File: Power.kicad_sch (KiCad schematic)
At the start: 39 parts, among them IC1 ADP2301AUJZ-R7, IC2 ADP2301AUJZ-R7, Q1 AO3401A, U1 LM2842X, U6 XT30PW-F, U7 XT30PW-M, U9 LP5907QMFX-3.3Q1

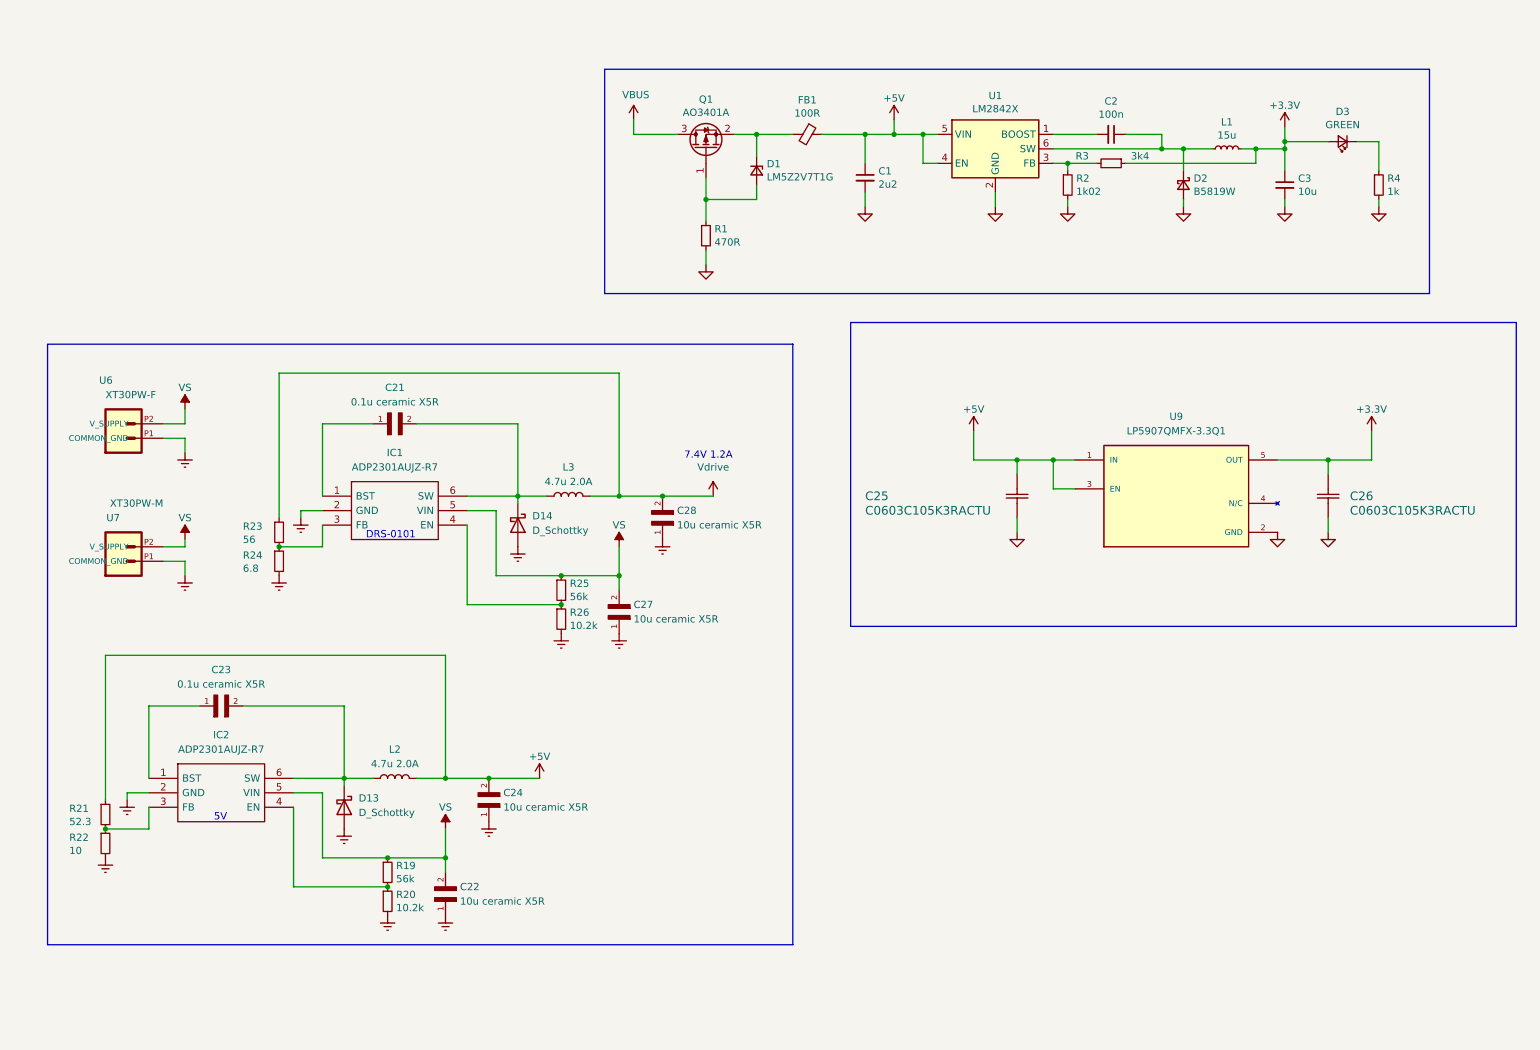
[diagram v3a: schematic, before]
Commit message: WEBGIOWEBGIOBWEG
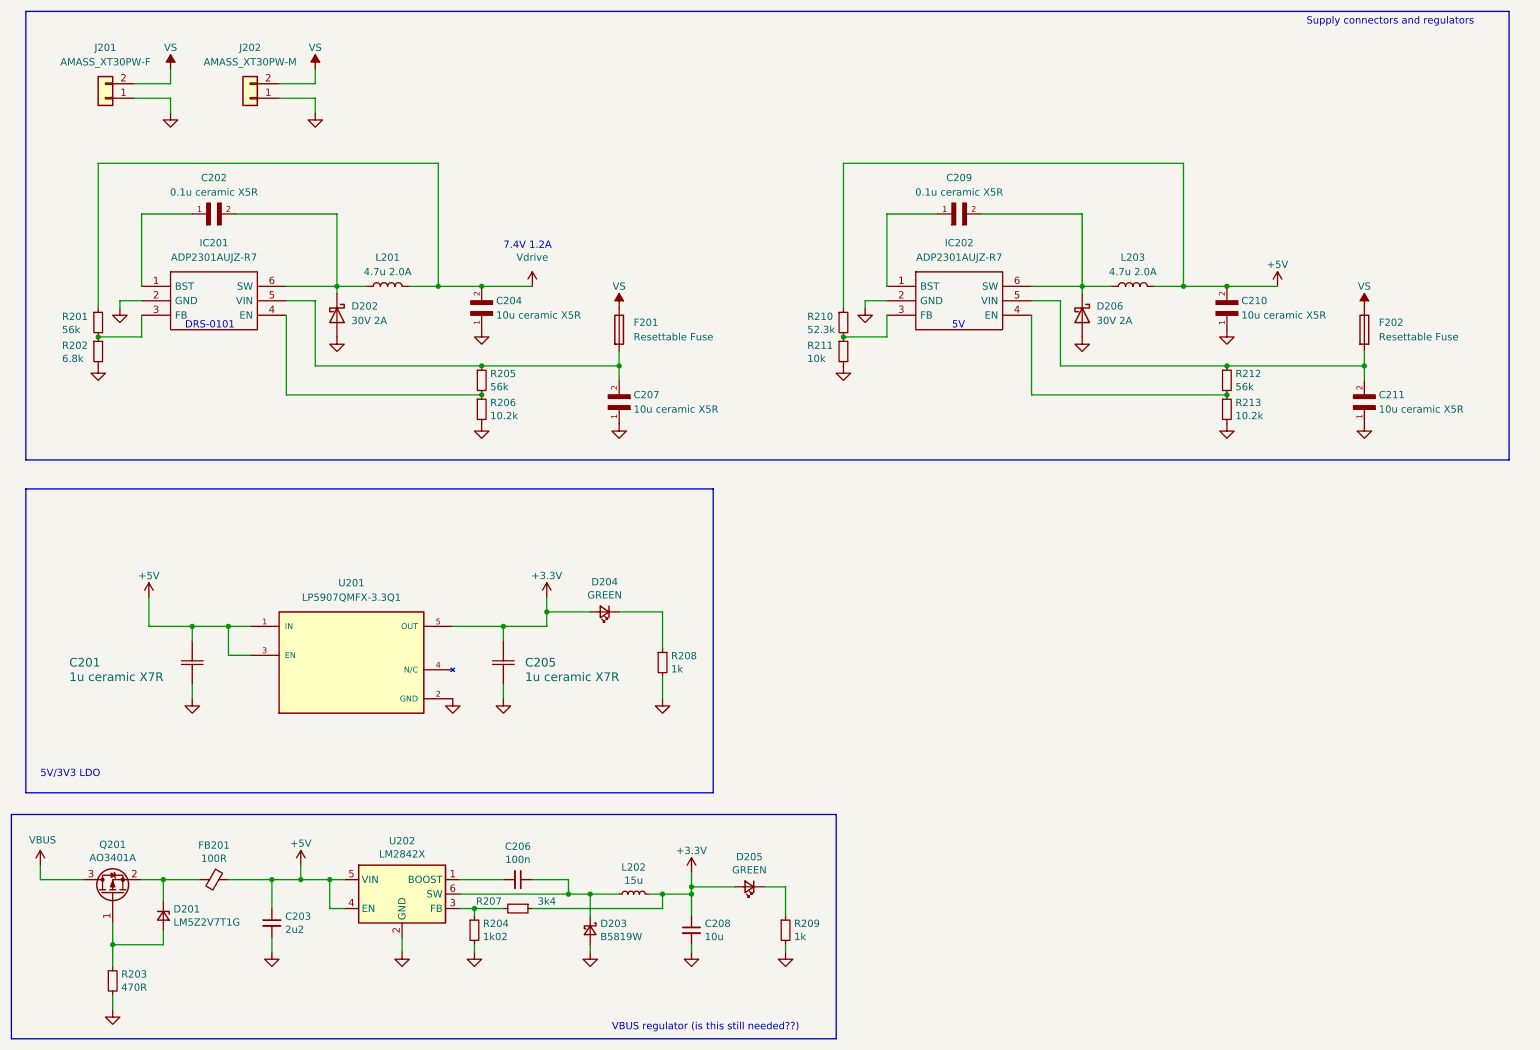
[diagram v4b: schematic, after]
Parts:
- removed C27: 10u ceramic X5R, SnapEDA Library:CAPC1608X90N, symbol C1608X5R0J106K080AB:C1608X5R0J106K080AB
- removed R25: 56k, Resistor_SMD:R_0402_1005Metric, symbol Device:R_Small
- removed R26: 10.2k, Resistor_SMD:R_0402_1005Metric, symbol Device:R_Small
- removed U6: XT30PW-F, Connector_AMASS:AMASS_XT30PW-F_1x02_P2.50mm_Horizontal, symbol XT30PW-F:XT30PW-F
- removed U7: XT30PW-M, Connector_AMASS:AMASS_XT30PW-M_1x02_P2.50mm_Horizontal, symbol XT30PW-F:XT30PW-F
- added C207: 10u ceramic X5R, SnapEDA Library:CAPC1608X90N, symbol C1608X5R0J106K080AB:C1608X5R0J106K080AB
- added D204: GREEN, LED_SMD:LED_0603_1608Metric, symbol Device:LED_Small
- added F201, F202: Resettable Fuse, symbol Device:Fuse
- added J201: AMASS_XT30PW-F, Connector_AMASS:AMASS_XT30PW-F_1x02_P2.50mm_Horizontal, symbol Connector_Generic:Conn_01x02
- added J202: AMASS_XT30PW-M, Connector_AMASS:AMASS_XT30PW-M_1x02_P2.50mm_Horizontal, symbol Connector_Generic:Conn_01x02
- added R205: 56k, Resistor_SMD:R_0402_1005Metric, symbol Device:R_Small
- added R206: 10.2k, Resistor_SMD:R_0402_1005Metric, symbol Device:R_Small
- added R208: 1k, Resistor_SMD:R_0402_1005Metric, symbol Device:R_Small
- C201: renamed from C25; value C0603C105K3RACTU -> 1u ceramic X7R
- C205: renamed from C26; value C0603C105K3RACTU -> 1u ceramic X7R
- D202: renamed from D14; value D_Schottky -> 30V 2A
- D206: renamed from D13; value D_Schottky -> 30V 2A
- L202: renamed from L1; footprint BluePhil-Footprints:MPIT4018-150M-LF -> BluePill-Footprints:MPIT4018-150M-LF
- R201: renamed from R23; value 56 -> 56k
- R202: renamed from R24; value 6.8 -> 6.8k
- R210: renamed from R21; value 52.3 -> 52.3k
- R211: renamed from R22; value 10 -> 10k
- renumbered C21 to C202, C1 to C203, C28 to C204, C2 to C206, C3 to C208, C23 to C209, C24 to C210, C22 to C211, D1 to D201, D2 to D203, D3 to D205, FB1 to FB201, IC1 to IC201, IC2 to IC202, L3 to L201, L2 to L203, Q1 to Q201, R1 to R203, R2 to R204, R3 to R207, R4 to R209, R19 to R212, R20 to R213, U9 to U201, U1 to U202
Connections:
- net Earth is gone; now on net GND: C204.1, C210.1, C211.1, D202.2 (A), D206.2 (A), IC201.2 (GND), IC202.2 (GND), R202.2, R211.2, R213.2
- net +3V3: now also D204.2 (A)
- net GND: now also C207.1, J201.1 (Pin_1), J202.1 (Pin_1), R206.2, R208.2
- net VS: now also F201.1, F202.1, J201.2 (Pin_2), J202.2 (Pin_2); no longer C211.2, IC201.5 (VIN), IC202.5 (VIN), R212.1
- net at IC201.4 (EN): now also R205.2, R206.1
- new net: C211.2, F202.2, IC202.5 (VIN), R212.1
- new net: D204.1 (K), R208.1
- new net: C207.2, F201.2, IC201.5 (VIN), R205.1
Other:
- note added: "5V/3V3 LDO"
- note added: "Supply connectors and regulators"
- note added: "VBUS regulator (is this still needed??)"
- moved on the sheet: C201, C202, C203, C204, C205, C206, C208, C209, C210, C211, D201, D202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
